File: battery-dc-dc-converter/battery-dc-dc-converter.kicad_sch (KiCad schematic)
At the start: 24 parts, among them J1 Conn_01x02, J2 Conn_01x01, J3 Conn_01x01, U1 LMR16030P

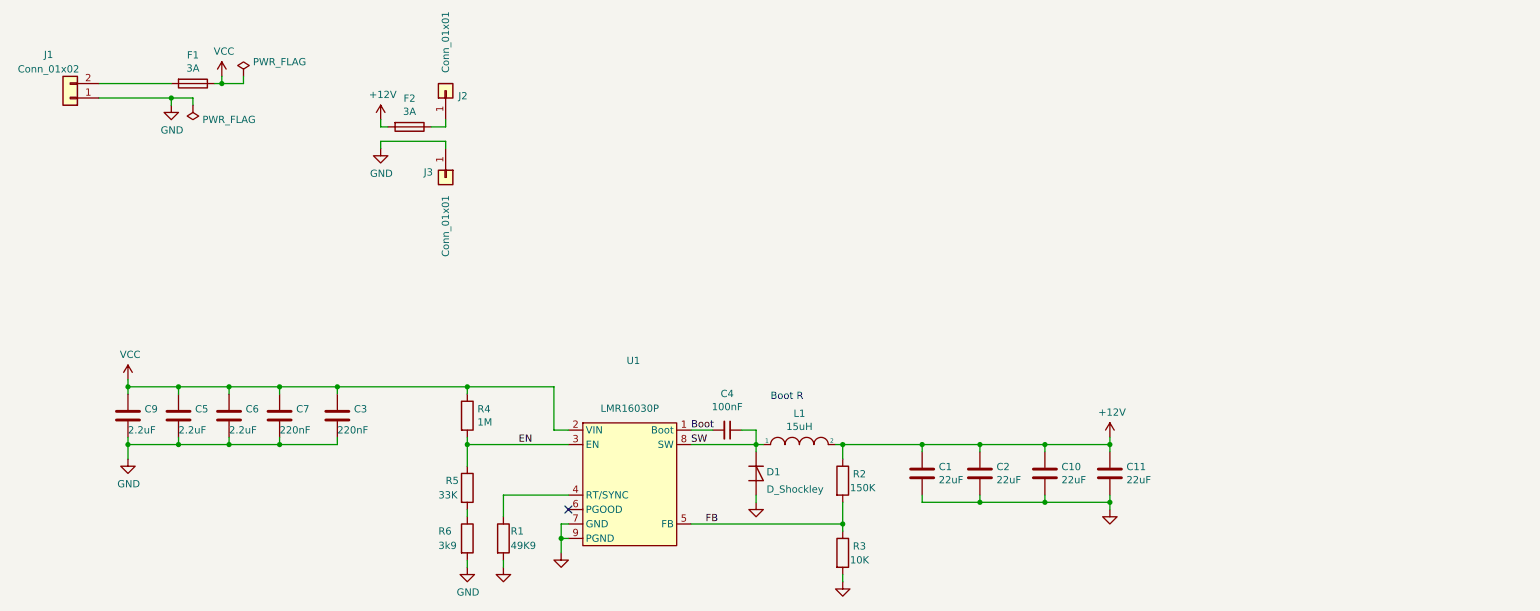
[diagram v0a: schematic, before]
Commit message: Tidy up
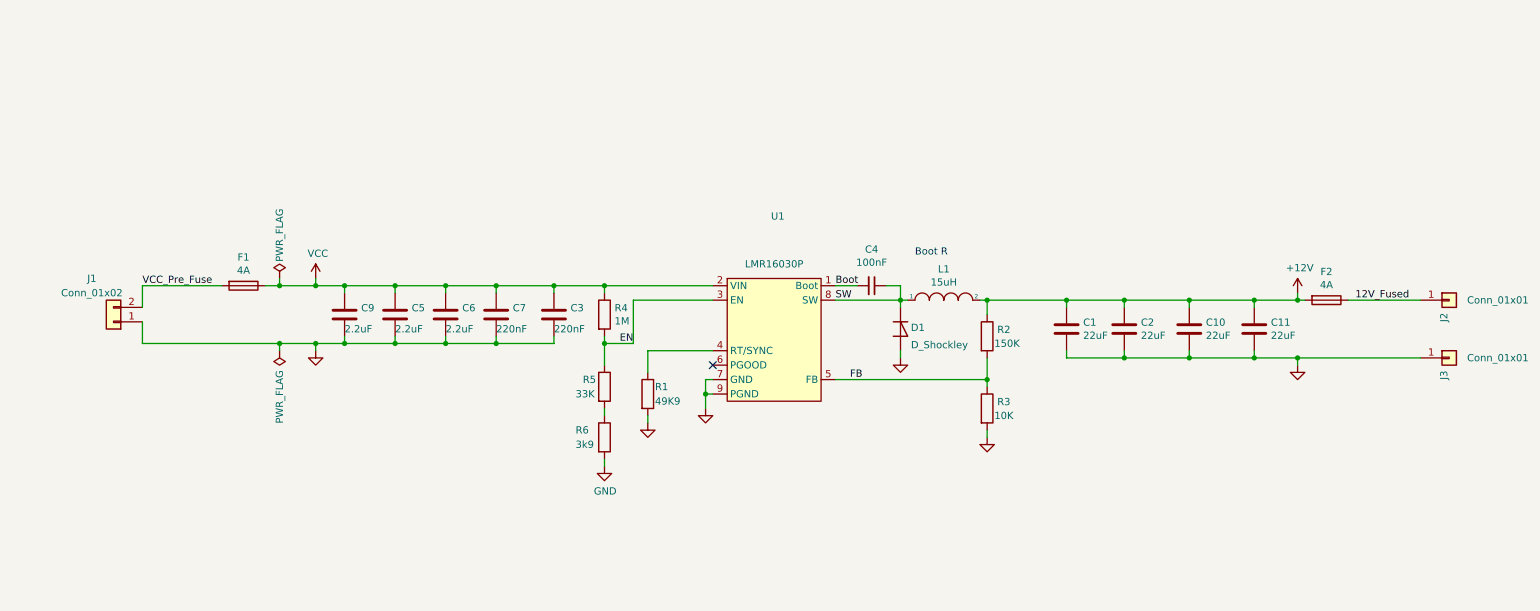
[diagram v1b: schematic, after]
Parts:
- F1, F2: value 3A -> 4A; LCSC C140478 -> C136349
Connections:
- net VCC_Pre_Fuse: now reaches F1.2, J1.2 (Pin_2)
- net 12V_Fused: now reaches F2.1, J2.1 (Pin_1)
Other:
- moved on the sheet: C1, C10, C11, C2, C3, C4, C5, C6, C7, C9, D1, F1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
